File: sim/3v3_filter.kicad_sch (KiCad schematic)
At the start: 7 parts

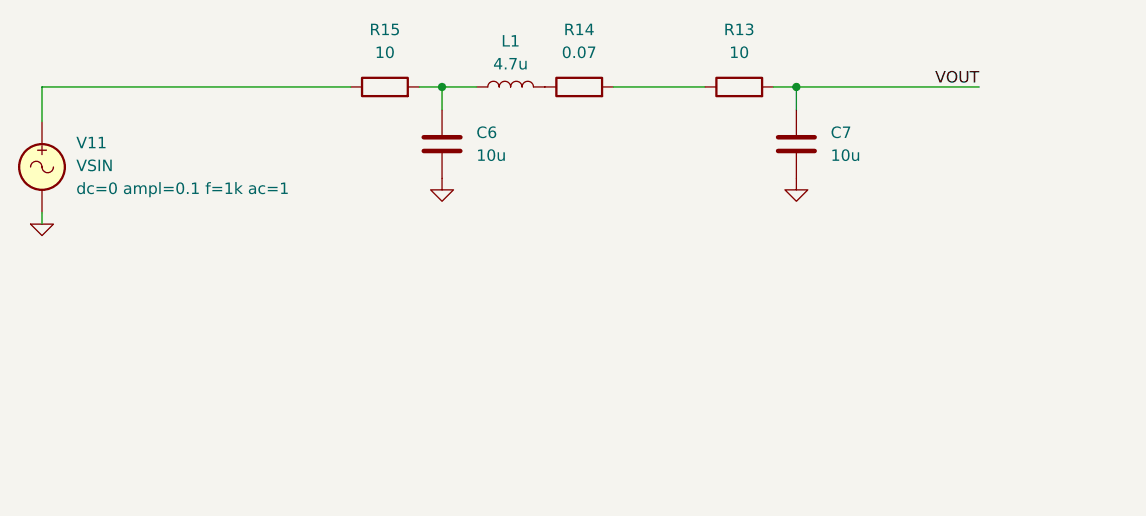
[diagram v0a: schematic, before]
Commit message: Routing almost finished
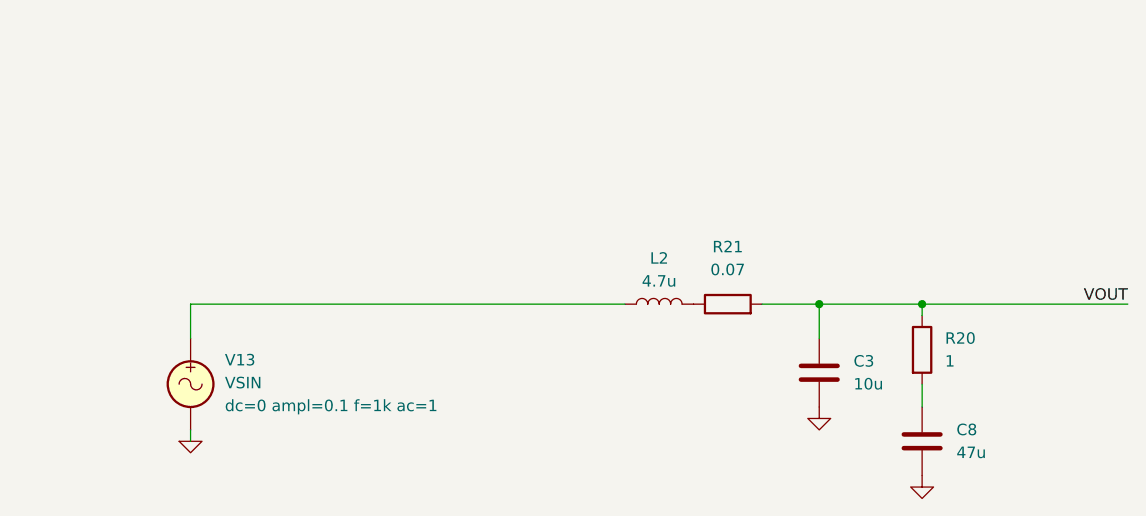
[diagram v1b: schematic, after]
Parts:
- removed C6, C7: 10u, Capacitor_SMD:C_1206_3216Metric, symbol Device:C
- removed L1: 4.7u, symbol Device:L
- removed R13, R15: 10, Resistor_SMD:R_0603_1608Metric, symbol rflib:R
- removed R14: 0.07, Resistor_SMD:R_0603_1608Metric, symbol rflib:R
- removed V11: VSIN, symbol Simulation_SPICE:VSIN
- added C3: 10u, Capacitor_SMD:C_1206_3216Metric, symbol Device:C
- added C8: 47u, Capacitor_SMD:C_1206_3216Metric, symbol Device:C
- added L2: 4.7u, symbol Device:L
- added R20: 1, symbol Device:R
- added R21: 0.07, Resistor_SMD:R_0603_1608Metric, symbol rflib:R
- added V13: VSIN, symbol Simulation_SPICE:VSIN
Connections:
- net 0: now also V13.2
- net GND: now also C3.2, C8.2
- net VOUT: now also C3.1, R20.1, R21.2
- new net: L2.1, V13.1
- new net: L2.2, R21.1
- new net: C8.1, R20.2
